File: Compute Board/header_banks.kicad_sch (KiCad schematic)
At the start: 28 parts, among them J10 Conn_01x03, J11 Conn_01x01, J13 Conn_01x18, J3 Conn_01x06, J4 Conn_02x06_Counter_Clockwise, J5 Conn_01x08, J6 Conn_01x07, J7 Conn_01x09, J8 Conn_01x09, J9 Conn_01x08, U12 TCA9546AD

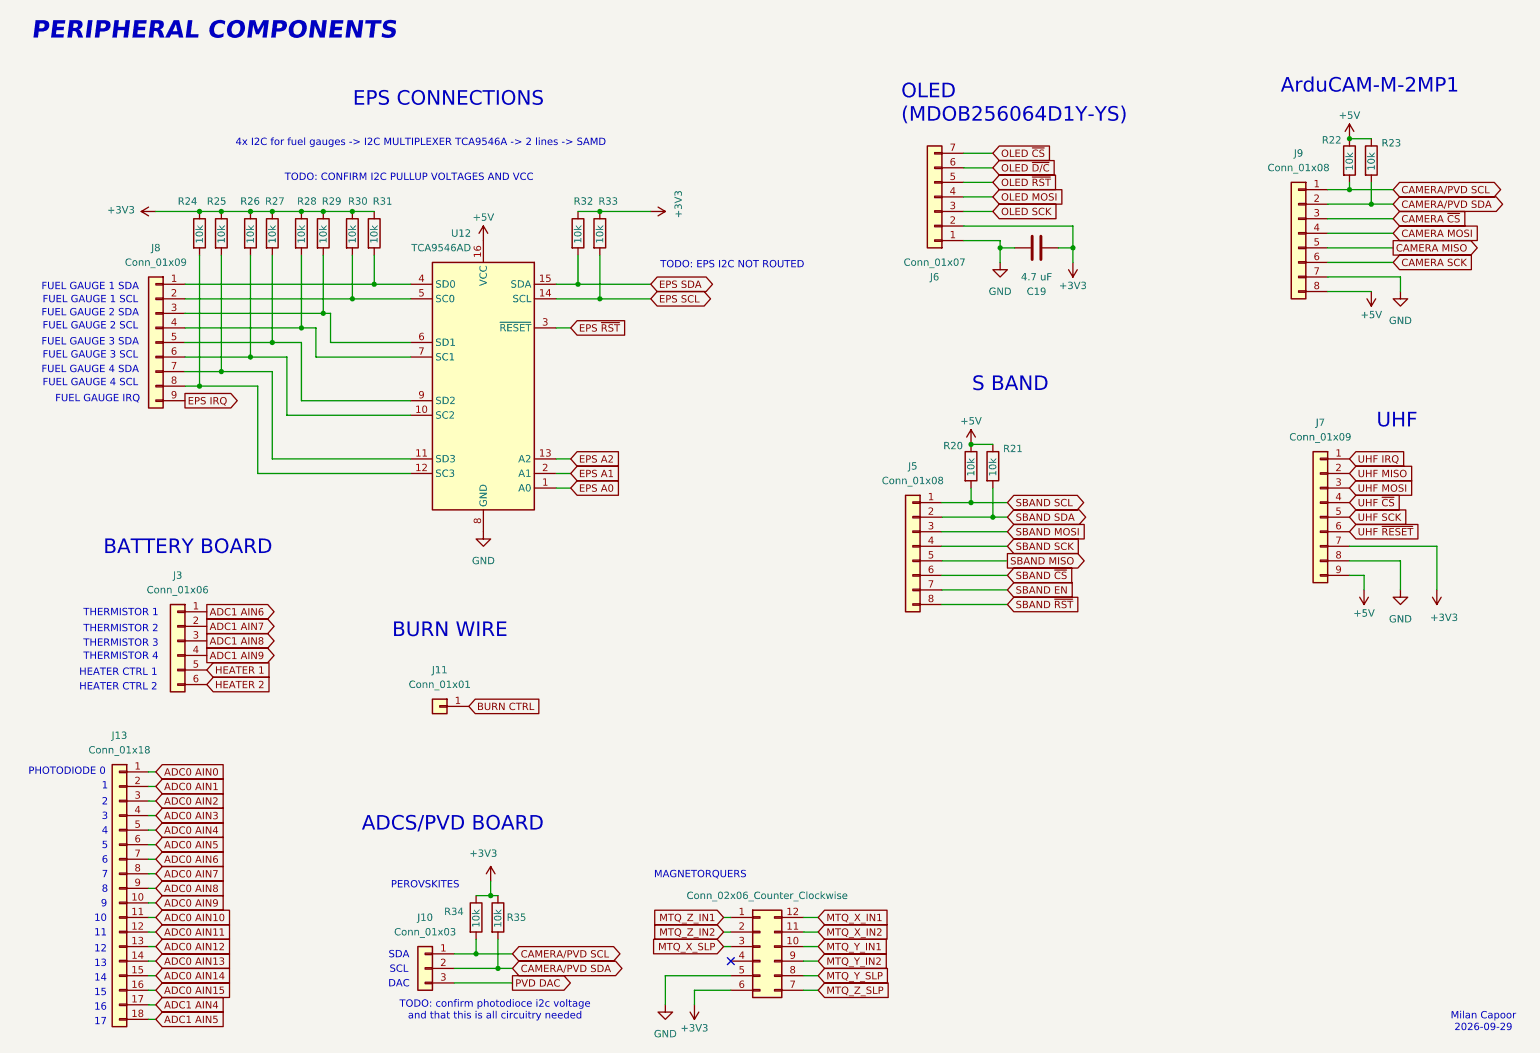
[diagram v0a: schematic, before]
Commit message: Finished routing
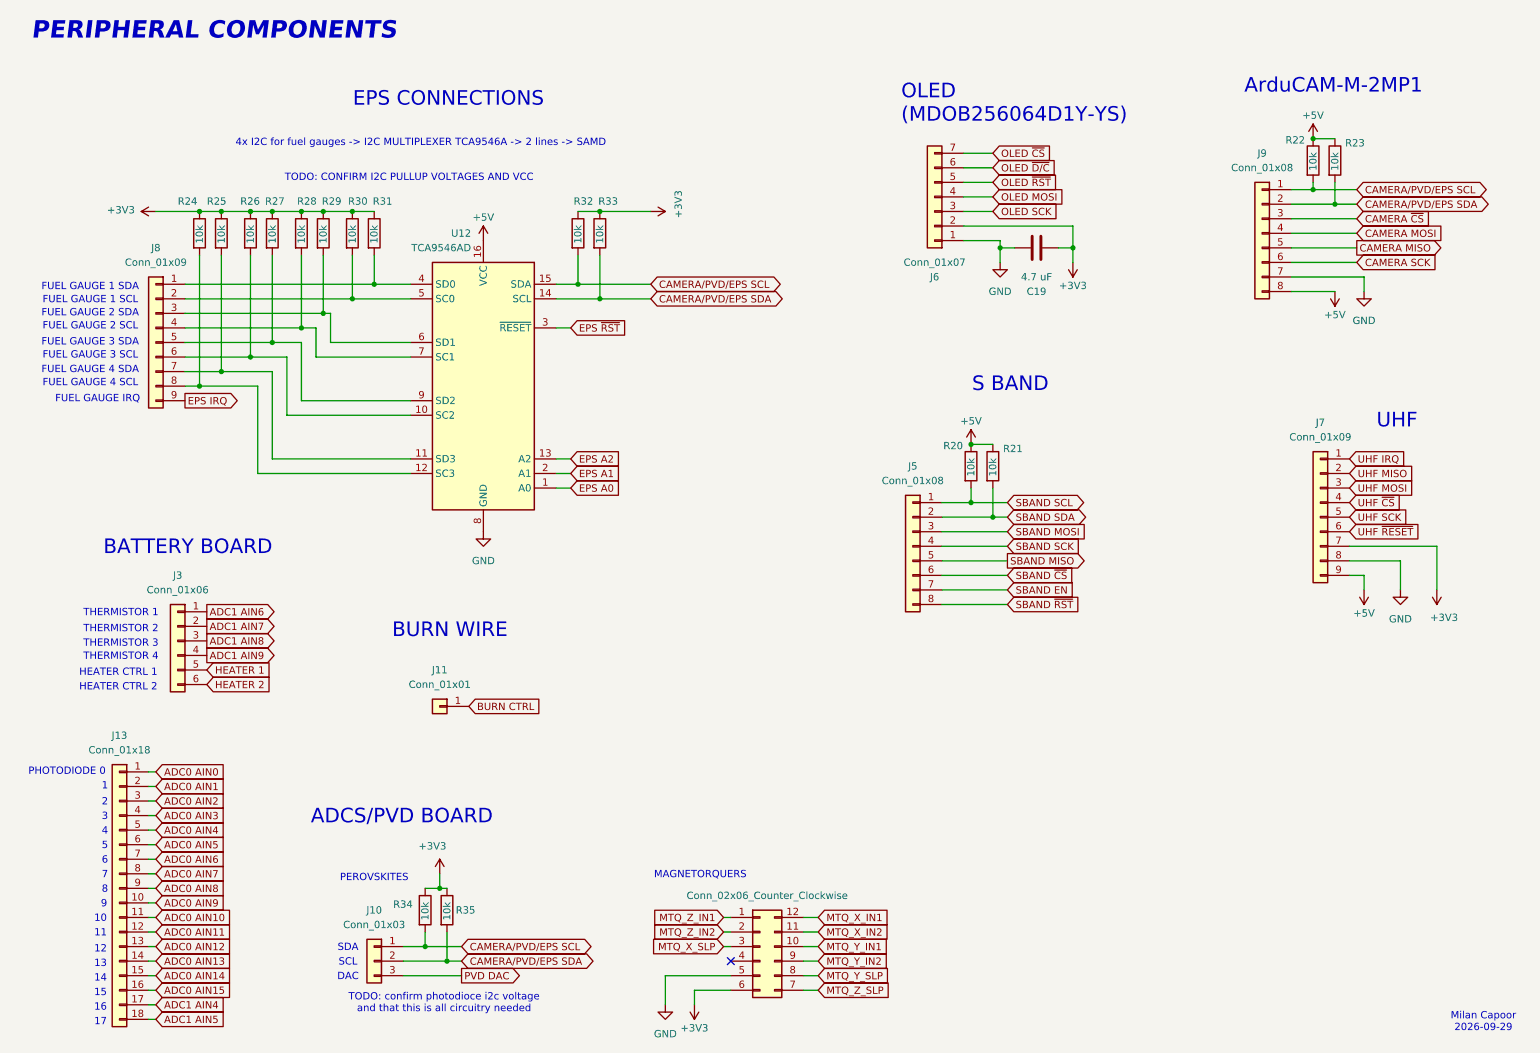
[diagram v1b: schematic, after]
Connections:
- net EPS SCL is gone; now on net CAMERA/PVD/EPS SDA: R33.2, U12.14 (SCL)
- net EPS SDA is gone; now on net CAMERA/PVD/EPS SCL: R32.2, U12.15 (SDA)
- net CAMERA/PVD SCL renamed CAMERA/PVD/EPS SCL
- net CAMERA/PVD SDA renamed CAMERA/PVD/EPS SDA
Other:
- note removed: "TODO: EPS I2C NOT ROUTED"
- moved on the sheet: J10, J9, R22, R23, R34, R35
